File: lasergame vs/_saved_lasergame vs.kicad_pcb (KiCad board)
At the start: 2 copper layers, 68.5 x 102.5 mm, 23 parts, among them J7 Programming port, Q1 IRLB8721PBF, SW2 SW_Reed, U1 ATmega328-PU, Y1 Crystal

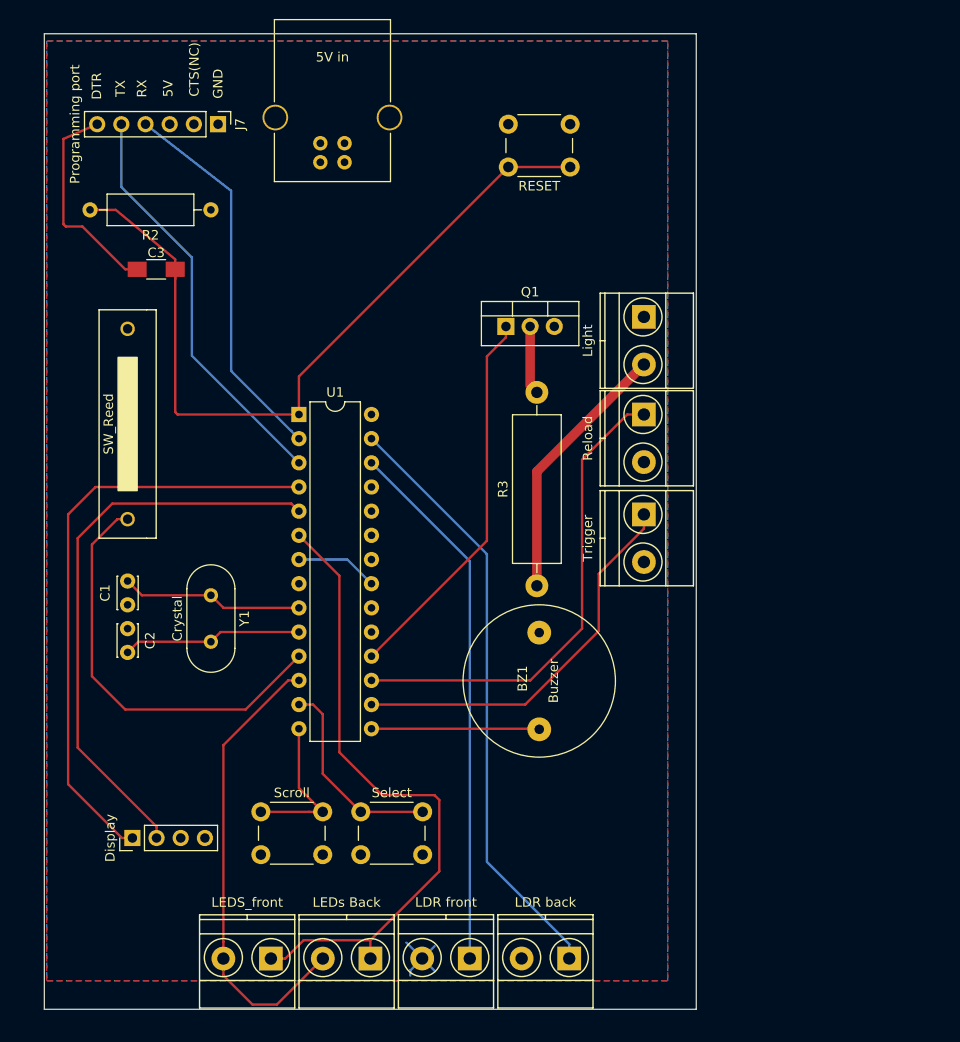
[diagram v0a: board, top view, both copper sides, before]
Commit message: first prototype pcb ordered
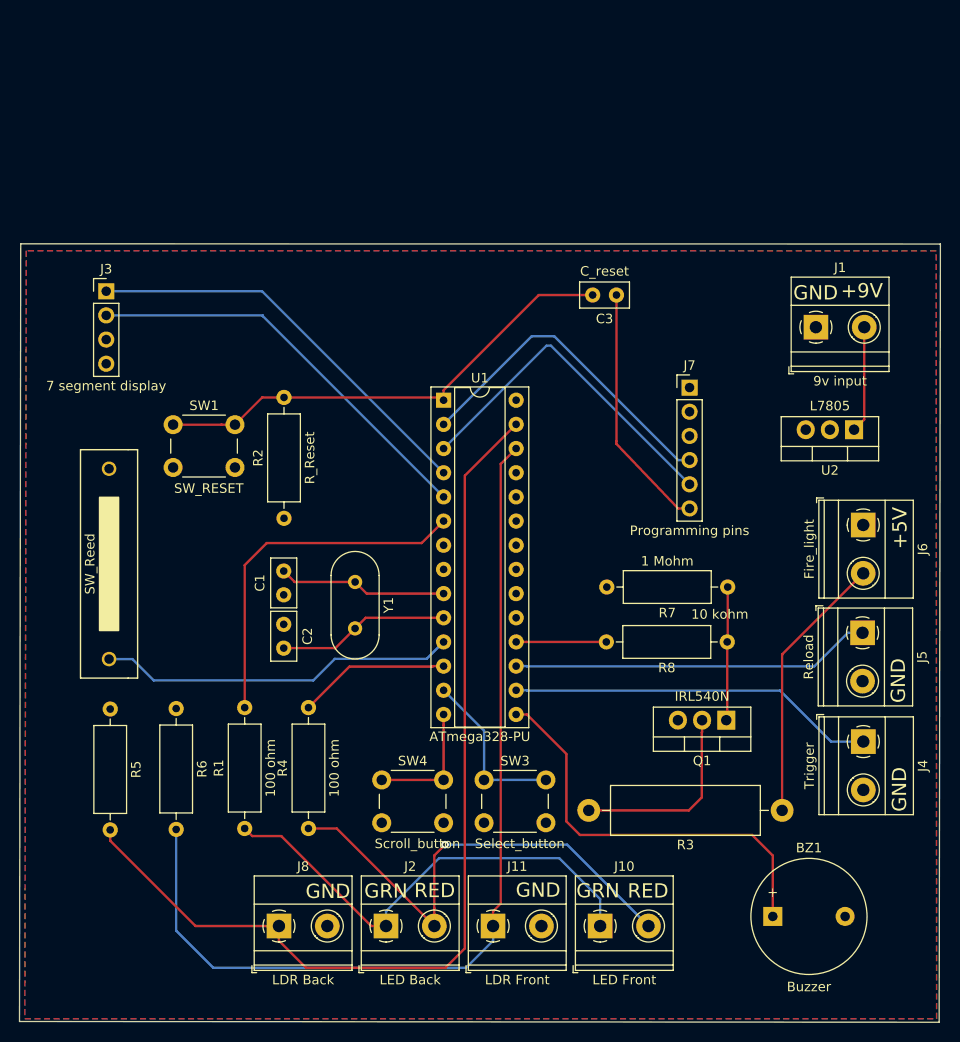
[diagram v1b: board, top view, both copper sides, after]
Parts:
- removed 5V in: USB_B, Connectors:USB_B
- removed Display: Conn_01x04_Female, Pin_Headers:Pin_Header_Straight_1x04_Pitch2.54mm
- removed LDR back: Screw_Terminal_01x02, TerminalBlocks_Phoenix:TerminalBlock_Phoenix_MKDS1.5-2pol
- removed LDR front: Screw_Terminal_01x02, TerminalBlocks_Phoenix:TerminalBlock_Phoenix_MKDS1.5-2pol
- removed LEDS_front, Light, Reload, Trigger: Screw_Terminal_01x02, TerminalBlocks_Phoenix:TerminalBlock_Phoenix_MKDS1.5-2pol
- removed LEDs Back: LED, TerminalBlocks_Phoenix:TerminalBlock_Phoenix_MKDS1.5-2pol
- removed RESET, Scroll, Select: SW_SPST, Buttons_Switches_THT:SW_PUSH_6mm_h9.5mm
- added J1: 9v input, TerminalBlock_Phoenix:TerminalBlock_Phoenix_MKDS-1,5-2-5.08_1x02_P5.08mm_Horizontal, F.Cu at (184.6, 70.8)
- added J10: LED Front, TerminalBlock_Phoenix:TerminalBlock_Phoenix_MKDS-1,5-2-5.08_1x02_P5.08mm_Horizontal, F.Cu at (161.9, 133.8)
- added J11: LDR Front, TerminalBlock_Phoenix:TerminalBlock_Phoenix_MKDS-1,5-2-5.08_1x02_P5.08mm_Horizontal, F.Cu at (150.7, 133.8)
- added J2: LED Back, TerminalBlock_Phoenix:TerminalBlock_Phoenix_MKDS-1,5-2-5.08_1x02_P5.08mm_Horizontal, F.Cu at (139.4, 133.8)
- added J3: 7 segment display, Connector_PinHeader_2.54mm:PinHeader_1x04_P2.54mm_Vertical, F.Cu at (110.0, 67.0)
- added J4: Trigger, TerminalBlock_Phoenix:TerminalBlock_Phoenix_MKDS-1,5-2-5.08_1x02_P5.08mm_Horizontal, F.Cu at (189.6, 114.4)
- added J5: Reload, TerminalBlock_Phoenix:TerminalBlock_Phoenix_MKDS-1,5-2-5.08_1x02_P5.08mm_Horizontal, F.Cu at (189.5, 102.9)
- added J6: Fire_light, TerminalBlock_Phoenix:TerminalBlock_Phoenix_MKDS-1,5-2-5.08_1x02_P5.08mm_Horizontal, F.Cu at (189.5, 91.6)
- added J8: LDR Back, TerminalBlock_Phoenix:TerminalBlock_Phoenix_MKDS-1,5-2-5.08_1x02_P5.08mm_Horizontal, F.Cu at (128.2, 133.8)
- added R1: 100 ohm, Resistor_THT:R_Axial_DIN0309_L9.0mm_D3.2mm_P12.70mm_Horizontal, F.Cu at (124.5, 123.5)
- added R4: 100 ohm, Resistor_THT:R_Axial_DIN0309_L9.0mm_D3.2mm_P12.70mm_Horizontal, F.Cu at (131.2, 123.5)
- added R5: R, Resistor_THT:R_Axial_DIN0309_L9.0mm_D3.2mm_P12.70mm_Horizontal, F.Cu at (110.4, 111.0)
- added R6: R, Resistor_THT:R_Axial_DIN0309_L9.0mm_D3.2mm_P12.70mm_Horizontal, F.Cu at (117.3, 110.9)
- added R7: 1 Mohm, Resistor_THT:R_Axial_DIN0309_L9.0mm_D3.2mm_P12.70mm_Horizontal, F.Cu at (175.3, 98.1)
- added R8: 10 kohm, Resistor_THT:R_Axial_DIN0309_L9.0mm_D3.2mm_P12.70mm_Horizontal, F.Cu at (175.2, 103.9)
- added SW1: SW_RESET, Button_Switch_THT:SW_PUSH_6mm_H9.5mm, F.Cu at (117.0, 81.1)
- added SW3: Select_button, Button_Switch_THT:SW_PUSH_6mm_H9.5mm, F.Cu at (149.7, 118.4)
- added SW4: Scroll_button, Button_Switch_THT:SW_PUSH_6mm_H9.5mm, F.Cu at (138.9, 118.4)
- added U2: L7805, Package_TO_SOT_THT:TO-220-3_Vertical, F.Cu at (188.6, 81.6)
- BZ1: footprint Buzzers_Beepers:BUZZER -> Buzzer_Beeper:Buzzer_12x9.5RM7.6
- C1, C2: footprint Capacitors_THT:C_Disc_D3.4mm_W2.1mm_P2.50mm -> Capacitor_THT:C_Disc_D5.0mm_W2.5mm_P2.50mm
- C3: value C -> C_reset; footprint Capacitors_SMD:C_1206_HandSoldering -> Capacitor_THT:C_Disc_D5.0mm_W2.5mm_P2.50mm
- J7: value Programming port -> Programming pins; footprint Pin_Headers:Pin_Header_Straight_1x06_Pitch2.54mm -> Connector_PinHeader_2.54mm:PinHeader_1x06_P2.54mm_Vertical
- Q1: value IRLB8721PBF -> IRL540N; footprint TO_SOT_Packages_THT:TO-220-3_Vertical -> Package_TO_SOT_THT:TO-220-3_Vertical
- R2: value R -> R_Reset; footprint Resistors_THT:R_Axial_DIN0309_L9.0mm_D3.2mm_P12.70mm_Horizontal -> Resistor_THT:R_Axial_DIN0309_L9.0mm_D3.2mm_P12.70mm_Horizontal
- R3: footprint Resistors_THT:R_Axial_DIN0516_L15.5mm_D5.0mm_P20.32mm_Horizontal -> Resistor_THT:R_Axial_DIN0516_L15.5mm_D5.0mm_P20.32mm_Horizontal
- U1: footprint Housings_DIP:DIP-28_W7.62mm -> Package_DIP:DIP-28_W7.62mm_Socket
- Y1: footprint Crystals:Crystal_HC49-U_Vertical -> Crystal:Crystal_HC49-U_Vertical
- moved J7 56.8 mm to (171.3, 77.2), turned to 0 degrees
- moved C3 48.4 mm to (163.6, 67.5), turned to 180 degrees
- moved Q1 47.4 mm to (175.2, 112.1), turned to 180 degrees
- moved R3 34.9 mm to (181.0, 121.6), turned to 180 degrees
- moved BZ1 34.8 mm to (180.0, 132.7), turned to 0 degrees
- moved R2 33.3 mm to (128.7, 90.9), turned to 90 degrees
- moved C1 16.4 mm to (128.7, 99.0)
- moved C2 16.4 mm to (128.7, 102.0)
- moved U1 15.3 mm to (145.4, 78.5)
- moved Y1 15.2 mm to (136.2, 97.6)
- moved SW2 14.8 mm to (110.3, 95.7)
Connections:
- J7 pad 2: Net-(J7-Pad2) -> (no net)
- U1 pad 12: LED_RED -> Net-(R4-Pad2)
- U1 pad 18: Light -> Net-(R8-Pad2)
- U1 pad 19: Net-(U1-Pad19) -> (no net)
- U1 pad 23: Net-(U1-Pad23) -> (no net)
- U1 pad 24: Net-(U1-Pad24) -> (no net)
- U1 pad 25: Net-(U1-Pad25) -> (no net)
- U1 pad 28: Net-(U1-Pad28) -> (no net)
- U1 pad 6: LED_GREEN -> Net-(R1-Pad2)
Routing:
- net LDR_FRONT: track 56.4 -> 99.5 mm
- net LDR_BACK: track 63.2 -> 103.0 mm
- net Net-(R1-Pad2): track 0.00 -> 37.8 mm
- net resetpin: track 82.6 -> 50.6 mm
- net Light: track 40.5 -> 14.1 mm
- net Buzzer: track 17.7 -> 43.7 mm
- net Clock: track 62.9 -> 43.3 mm
- net LED_GREEN: track 68.0 -> 50.1 mm
- net DIO: track 60.0 -> 43.4 mm
- net Net-(R4-Pad2): track 0.00 -> 16.0 mm
- net Net-(Q1-Pad2): track 7.22 -> 20.6 mm
- net Reload: track 50.6 -> 37.9 mm
- net +9V: track 0.00 -> 11.2 mm
- net Net-(R8-Pad2): track 0.00 -> 9.48 mm
- net 5V: track 8.67 -> 0.00 mm
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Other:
- board size 68.5 x 102.5 mm -> 96.8 x 81.8 mm
- board text added: "+5V"
- board text added: "+9V"
- board text added: "GRN"
- board text added: "RED"
- board text removed: "5V"
- board text removed: "CTS(NC)"
- board text removed: "DTR"
- board text removed: "RX"
- board text removed: "TX"
